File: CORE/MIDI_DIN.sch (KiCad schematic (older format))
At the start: 61 parts, among them J1 Conn_02x08_Odd_Even, J2 USB_C_Receptacle_USB2.0, J3 Conn_01x04, J5 MAB5100S, J6 MAB5100S, J7 Conn_01x06, Q1 BSS84, Q2 BSS84, SW1 SW_SPDT, SW2 SW_Push_DPDT, SW3 PROG, SW4 SW_DIP_x04, SW5 RST, U1 ATSAMD21G15B-A, U2 H11L1, U3 MIC5504-3.3YM5, U4 MCP2517FD-xSL, U5 TLE9250V, Y1 20MHz

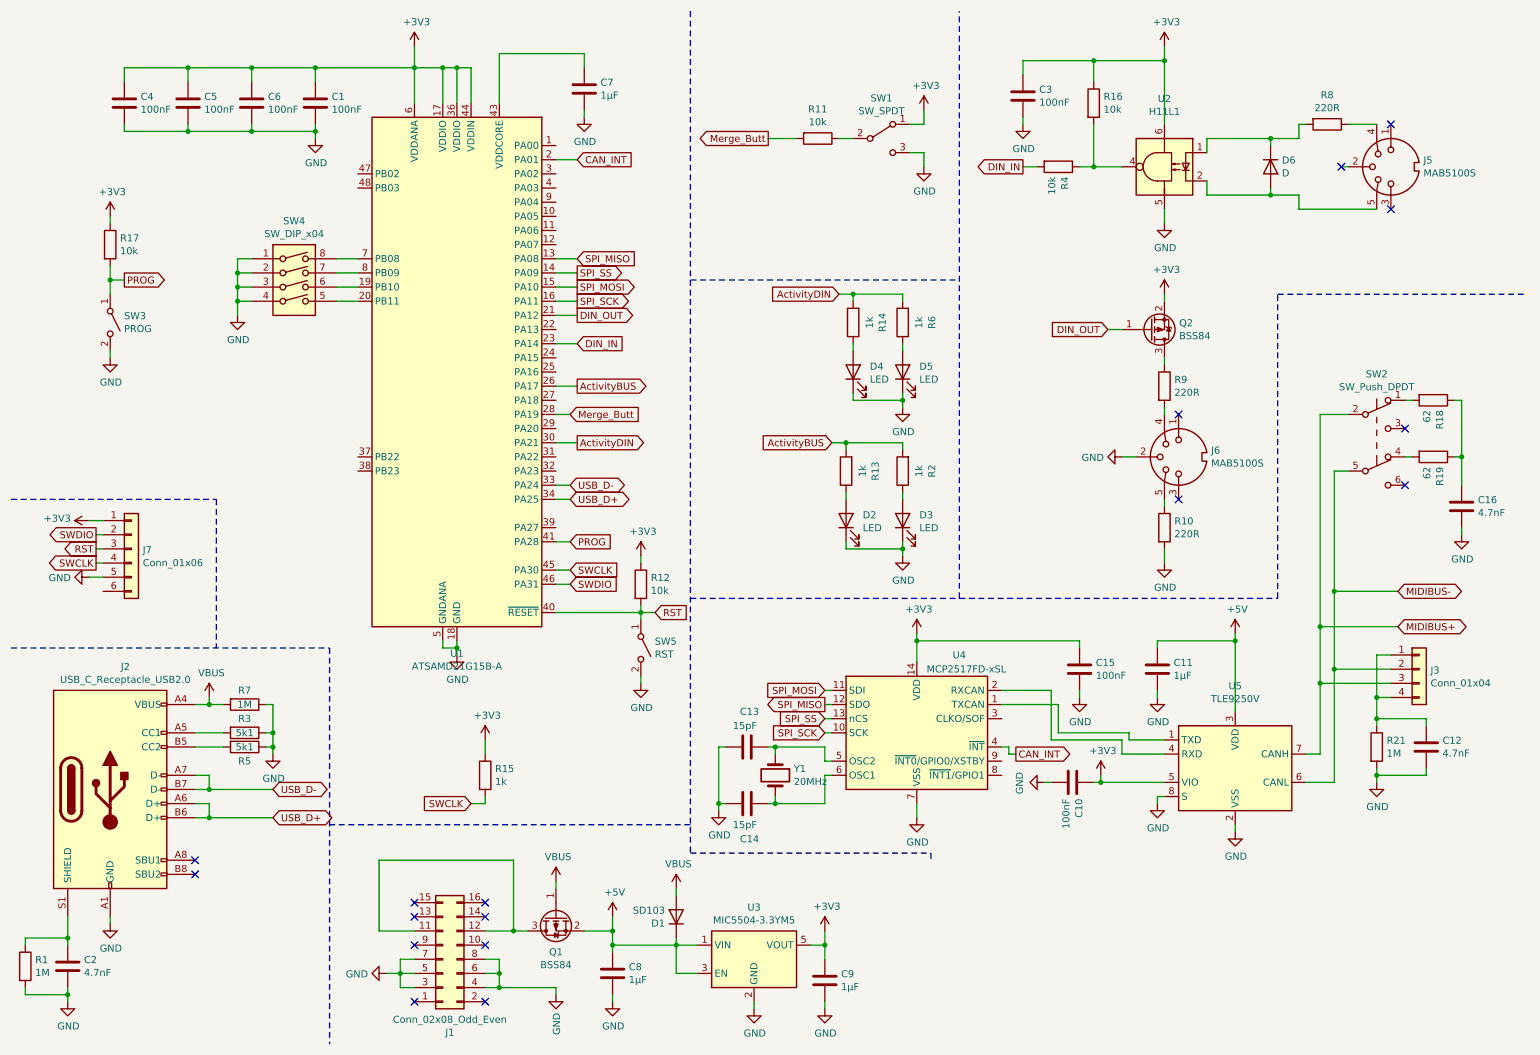
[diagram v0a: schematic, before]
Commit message: Rearrange and re-wire
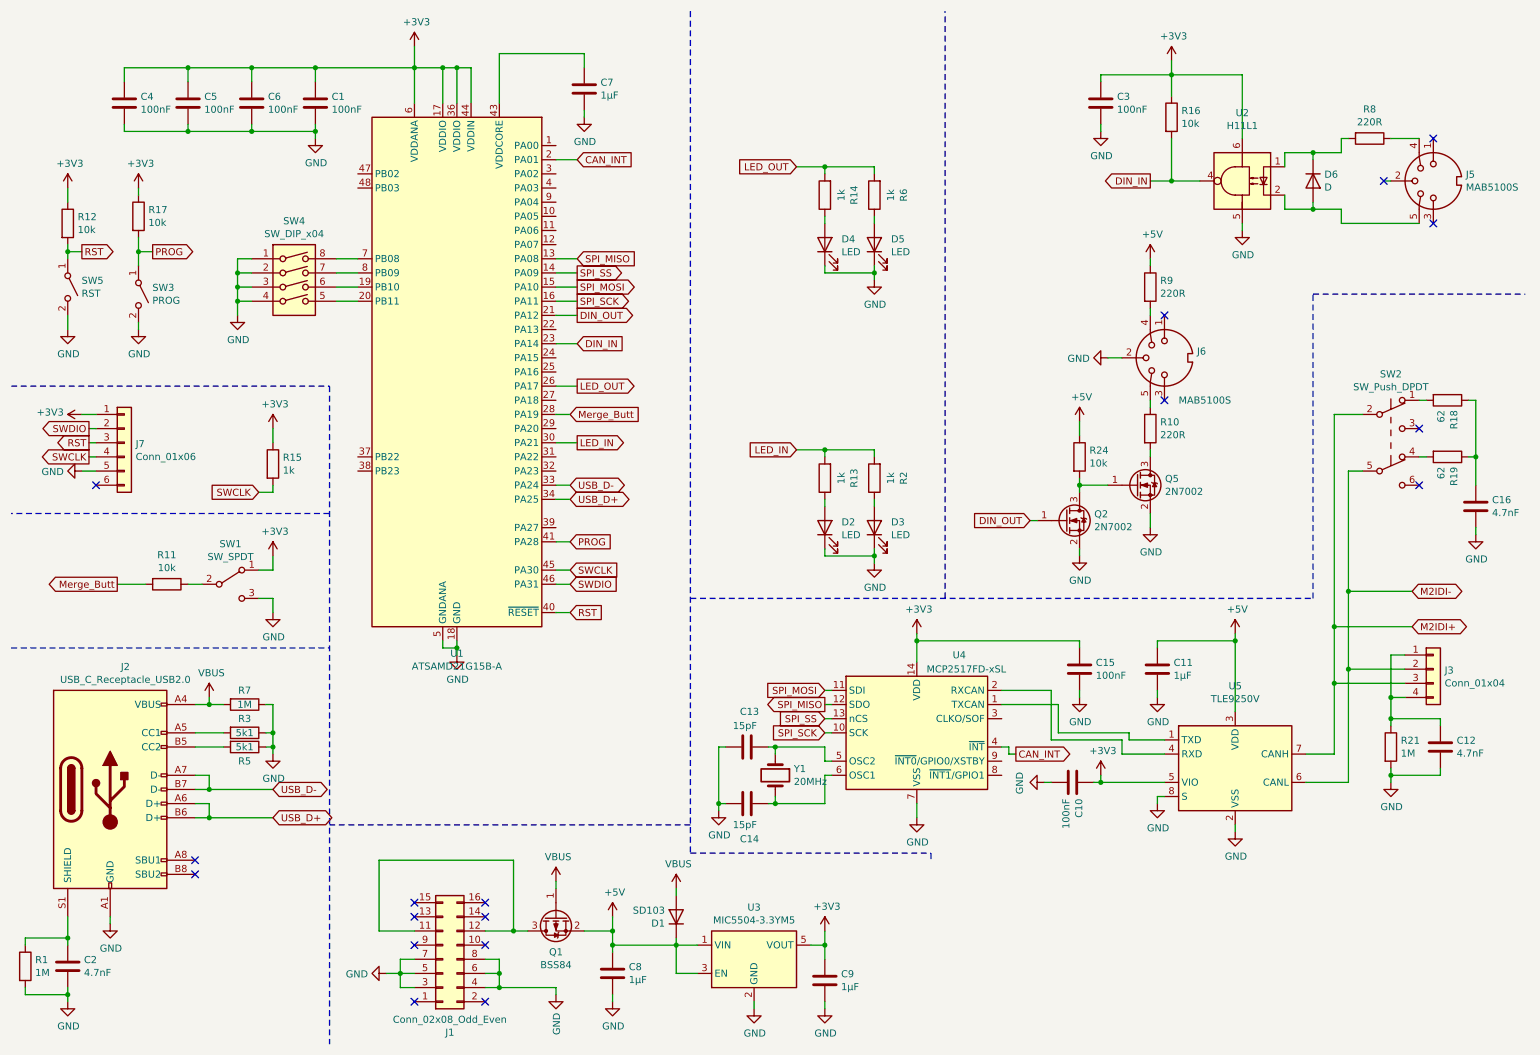
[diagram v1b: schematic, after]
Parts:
- removed Q2: BSS84, Package_TO_SOT_SMD:SOT-23, symbol Transistor_FET:BSS84
- removed R4: 10k, Resistor_SMD:R_0603_1608Metric, symbol Device:R
- added Q2, Q5: 2N7002, Package_TO_SOT_SMD:SOT-23, symbol Transistor_FET:2N7002
- added R24: 10k, Resistor_SMD:R_0603_1608Metric, symbol Device:R
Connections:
- net +5V: now also R9.1, R24.1
- net DIN_IN: now also R16.2, U2.4
- net DIN_OUT: now also Q2.1 (G)
- net GND: now also Q2.2 (S), Q5.2 (S); no longer R10.2
- net ActivityBUS renamed LED_IN
- net LED_IN: now also U1.30 (PA21); no longer U1.26 (PA17)
- net ActivityDIN renamed LED_OUT
- net LED_OUT: now also U1.26 (PA17); no longer U1.30 (PA21)
- net MIDIBUS+ renamed M2IDI+
- net MIDIBUS- renamed M2IDI-
- new net: Q5.3 (D), R10.2
- new net: Q2.3 (D), Q5.1 (G), R24.2
- no-connect marks 17 -> 18
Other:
- moved on the sheet: C12, C16, C3, D2, D3, D4, D5, D6, J3, J5, J6, J7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
